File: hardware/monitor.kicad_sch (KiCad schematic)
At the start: 1 part, among them U25 Teensy++2.0

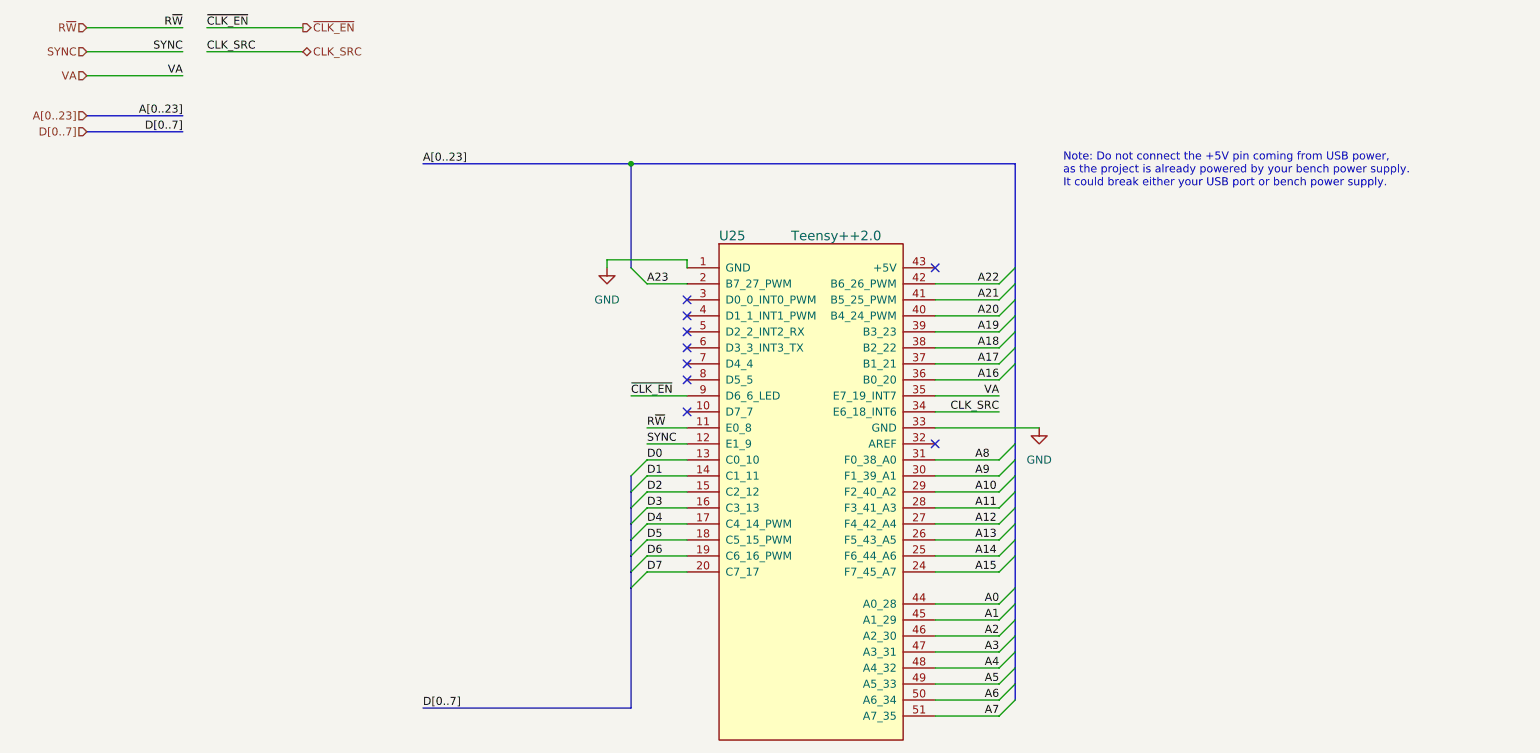
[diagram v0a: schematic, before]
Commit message: Prep ep 28
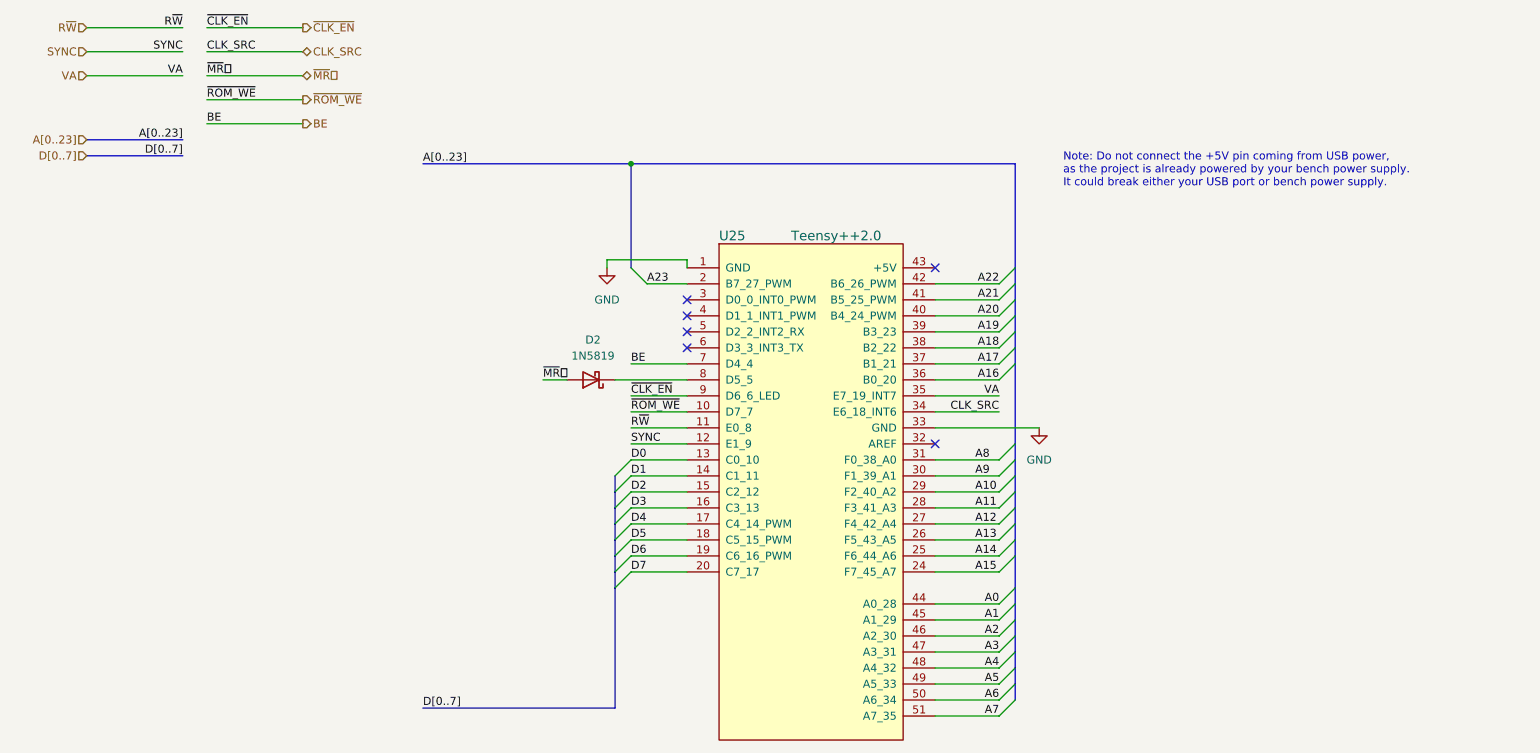
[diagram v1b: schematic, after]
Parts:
- added D2: 1N5819, Diode_THT:D_DO-41_SOD81_P10.16mm_Horizontal, symbol Diode:1N5819
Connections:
- net ~{ROM_WE}: now reaches U25.10 (D7_7)
- net BE: now reaches U25.7 (D4_4)
- net at U25.8 (D5_5): now also D2.1 (K)
- new net ~{MR}⎒: D2.2 (A)
- no-connect marks 9 -> 6
